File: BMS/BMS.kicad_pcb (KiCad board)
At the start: 2 copper layers, 69.4 x 69.4 mm, 97 parts, among them J1 Cell Taps, J10 IsoSPI, J2 IsoSPI, J3 Temp Sensors, Q1 NSV1C201MZ4, Q2 BSS308PE, Q3 BSS308PE, Q4 BSS308PE, Q5 BSS308PE, Q6 BSS308PE, Q7 BSS308PE, Q8 BSS308PE, SW1 SW_DIP_x04, U1 LTC6811, U2 ADG708

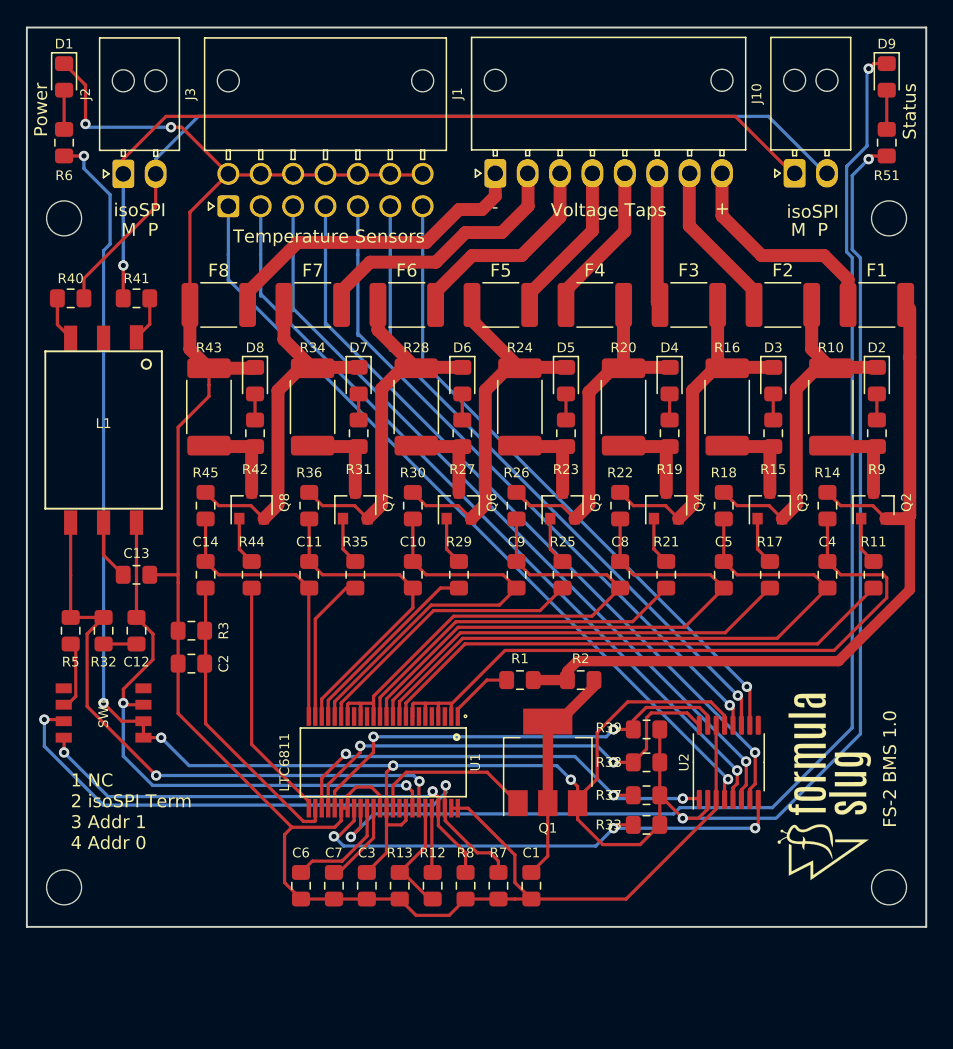
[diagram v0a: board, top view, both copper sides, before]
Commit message: Layout v1.1 of BMS
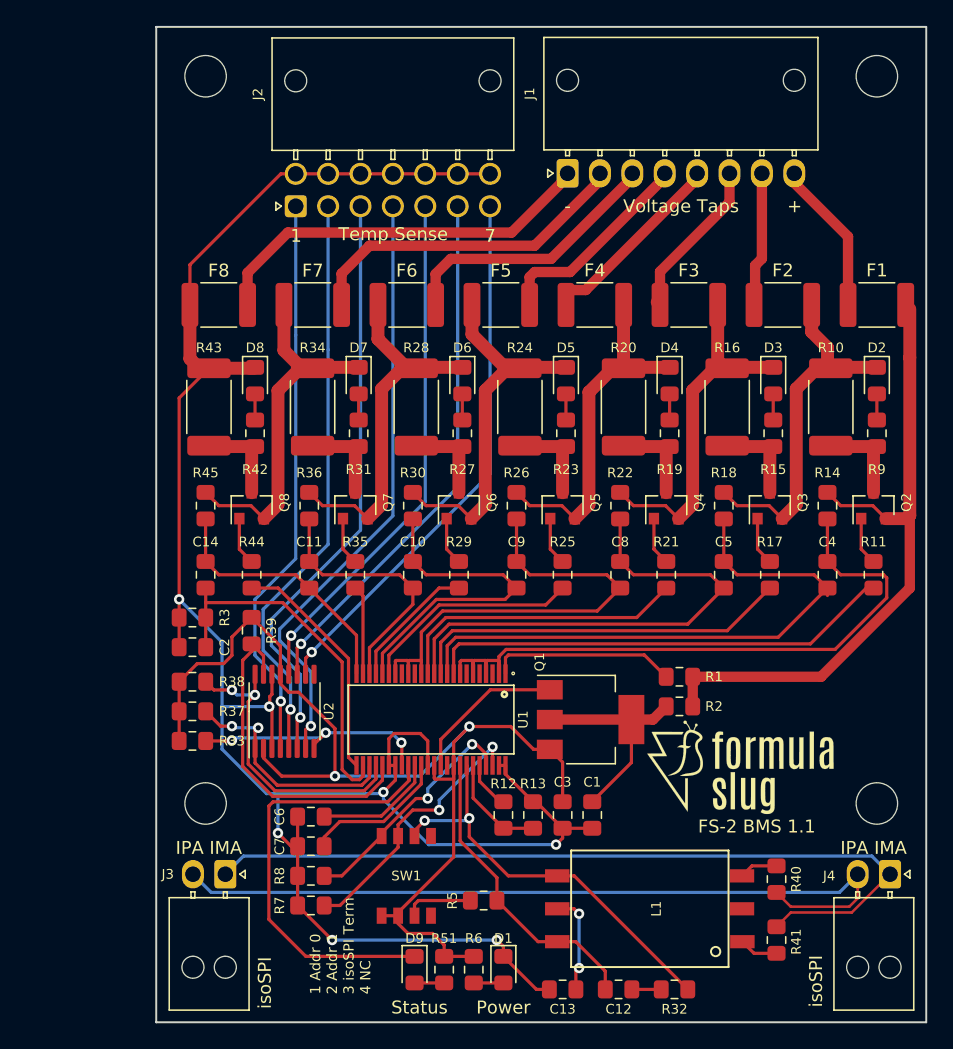
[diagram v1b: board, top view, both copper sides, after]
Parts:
- removed the ? at (90.9, 69.8)
- removed the ? at (90.9, 121.4)
- removed the ? at (154.6, 121.4)
- removed the ? at (154.7, 69.8)
- removed the J3 at (103.6, 68.8)
- added ?: MountingHole_3.2mm_M3, MountingHole:MountingHole_3.2mm_M3, F.Cu at (101.9, 114.9)
- added ?: MountingHole_3.2mm_M3, MountingHole:MountingHole_3.2mm_M3, F.Cu at (101.9, 58.8)
- added ?: MountingHole_3.2mm_M3, MountingHole:MountingHole_3.2mm_M3, F.Cu at (153.7, 58.8)
- added ?: MountingHole_3.2mm_M3, MountingHole:MountingHole_3.2mm_M3, F.Cu at (153.7, 114.9)
- added J2: Temp Sensors, Connector_Molex:Molex_Nano-Fit_105314-xx14_2x07_P2.50mm_Horizontal, F.Cu at (108.8, 68.8)
- moved D9 78.0 mm to (118.0, 127.8)
- moved D1 76.8 mm to (124.8, 127.8)
- moved R51 72.4 mm to (120.3, 127.8), turned to 90 degrees
- moved R6 71.2 mm to (122.6, 127.8), turned to 90 degrees
- moved R40 70.6 mm to (145.9, 120.8), turned to 90 degrees
- moved R41 70.0 mm to (145.9, 125.5), turned to 270 degrees
- moved L1 56.1 mm to (136.1, 123.1), turned to 90 degrees
- moved J3 54.6 mm to (103.4, 120.4), turned to 270 degrees
- moved J4 54.6 mm to (154.7, 120.4), turned to 270 degrees
- moved R32 52.0 mm to (138.0, 129.3), turned to 180 degrees
- moved C12 46.4 mm to (133.7, 129.3), turned to 0 degrees
- moved C13 45.9 mm to (129.4, 129.3), turned to 180 degrees
- moved R5 38.1 mm to (123.3, 122.4), turned to 180 degrees
- moved R33 35.6 mm to (100.8, 110.1), turned to 180 degrees
- moved R37 35.6 mm to (100.8, 107.8), turned to 180 degrees
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- renumbered J2 to J3, J10 to J4
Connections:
- net /IsoSPI_N renamed /extIsoSPI_N
- net /IsoSPI_P renamed /extIsoSPI_P
- C12 pad 1: IMA -> IsoSPI_N
- L1 pad 4: IPA -> IsoSPI_P
- L1 pad 6: IMA -> IsoSPI_N
- R32 pad 1: IPA -> IsoSPI_P
- R5 pad 1: Net-(R5-Pad1) -> IsoSPI_N
- R5 pad 2: IPA -> Net-(R5-Pad2)
- SW1 pad 2: Net-(R5-Pad1) -> IsoSPI_P
- SW1 pad 7: IMA -> Net-(R5-Pad2)
- U1 pad 41: IMA -> IsoSPI_N
- U1 pad 42: IPA -> IsoSPI_P
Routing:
- net VREG: track 202.9 -> 88.3 mm, vias 7 -> 2
- net Net-(D9-Pad1): track 98.0 -> 34.0 mm, vias 2 -> 0
- net IPA: track 47.4 -> 0.00 mm, vias 2 -> 0
- net IMA: track 45.8 -> 0.00 mm, vias 2 -> 0
- net IsoSPI_P: track 0.00 -> 32.4 mm, vias 0 -> 2
- net A1: track 46.5 -> 21.0 mm
- net IsoSPI_N: track 0.00 -> 23.6 mm
- net TEMP: track 40.4 -> 18.7 mm
- net A0: track 39.1 -> 18.5 mm
- net Net-(J2-Pad1): track 62.1 -> 44.0 mm
- net MUX_A0: track 35.2 -> 18.1 mm, vias 3 -> 2
- net Net-(J2-Pad2): track 61.3 -> 44.9 mm
- net Net-(J2-Pad3): track 60.6 -> 45.7 mm
- net Net-(J2-Pad4): track 59.9 -> 46.6 mm
- net MUX_A1: track 35.9 -> 23.5 mm
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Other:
- board size 69.4 x 69.4 mm -> 59.4 x 76.8 mm
- board text added: "1"
- board text added: "1 Addr 0 2 Addr 1 3 isoSPI Term 4 NC"
- board text added: "7"
- board text added: "FS-2 BMS 1.1"
- board text added: "IPA IMA"
- board text added: "Temp Sense"
- board text removed: "1 NC 2 isoSPI Term 3 Addr 1 4 Addr 0"
- board text removed: "FS-2 BMS 1.0"
- board text removed: "M P"
- board text removed: "Temperature Sensors"
